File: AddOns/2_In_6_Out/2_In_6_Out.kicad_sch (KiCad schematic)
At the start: 13 parts, among them J1 Heimtime, J2 MasterTrigger, J3 Conn_01x13_Socket, J4 Conn_01x04_Socket, J5 Conn_01x04_Socket

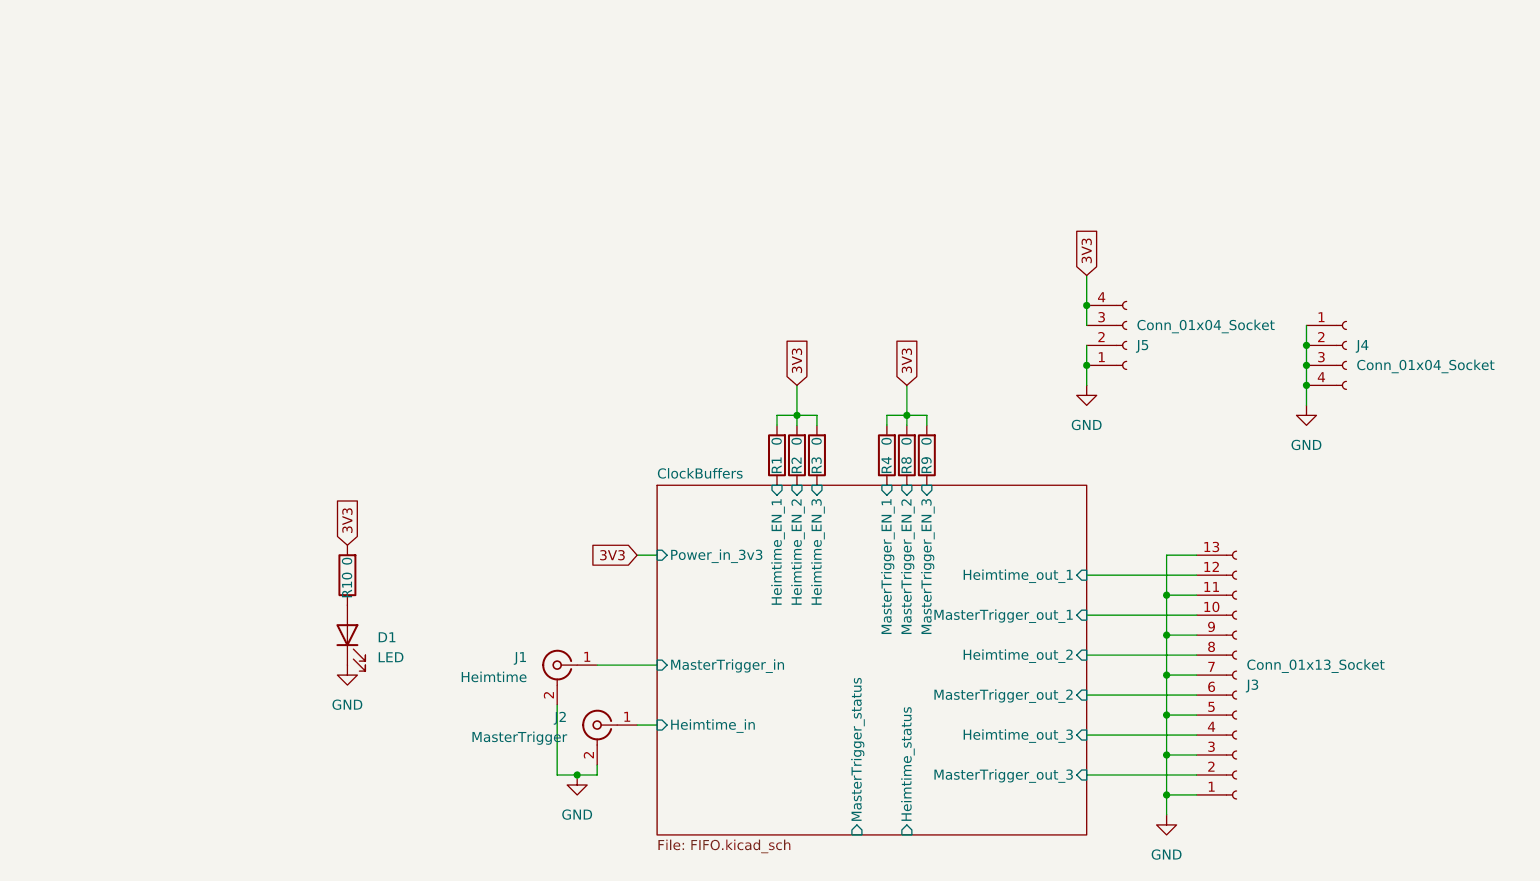
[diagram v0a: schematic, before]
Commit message: .
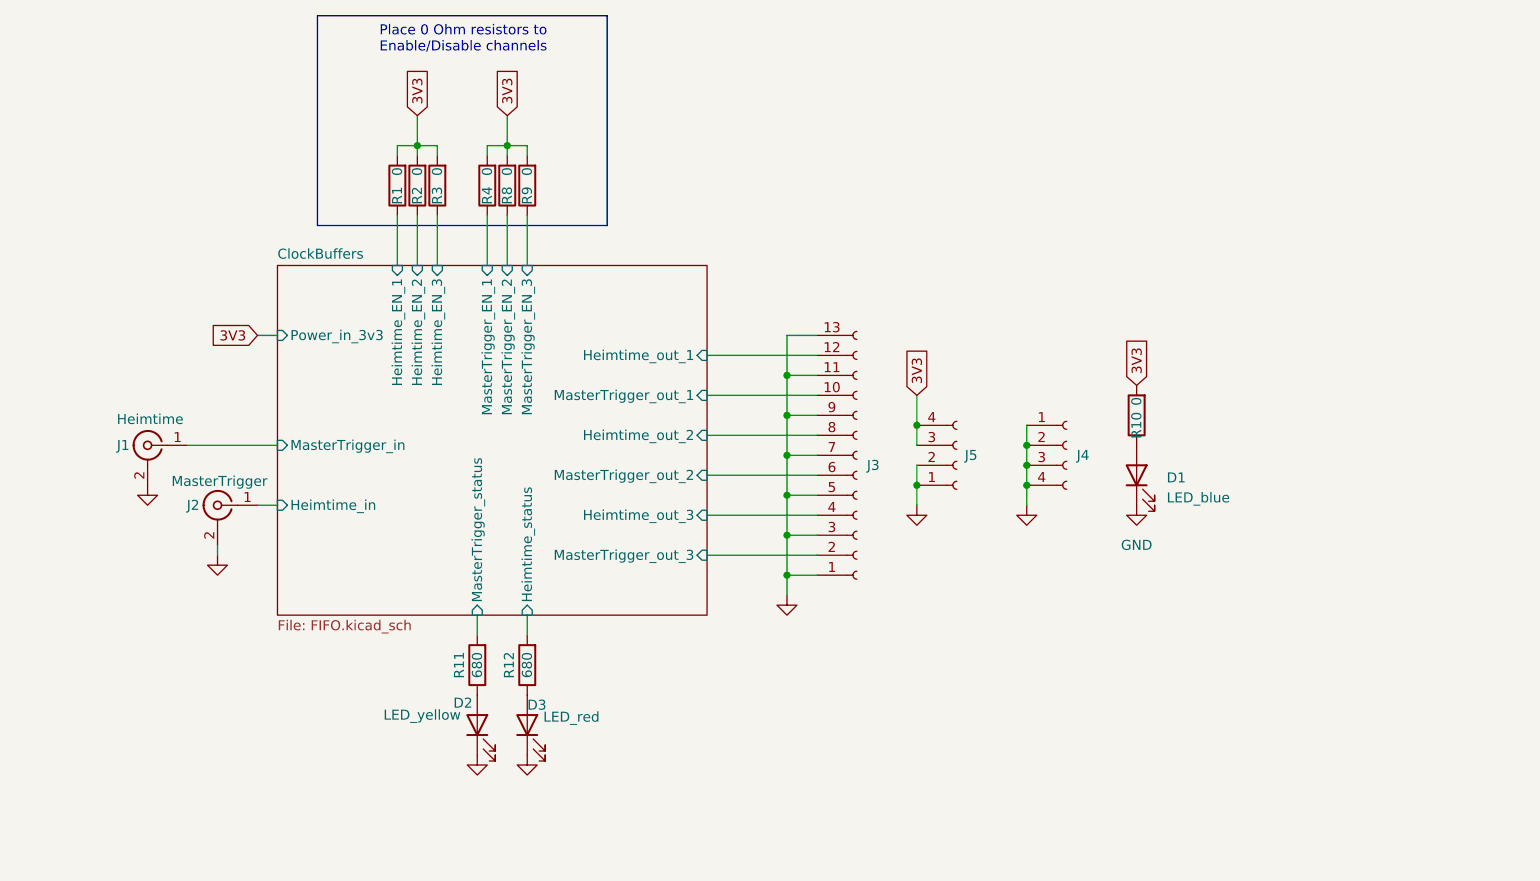
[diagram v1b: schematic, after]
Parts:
- added D2: LED_yellow, LED_SMD:LED_0603_1608Metric, symbol Device:LED
- added D3: LED_red, LED_SMD:LED_0603_1608Metric, symbol Device:LED
- added R11, R12: 680, Resistor_SMD:R_0402_1005Metric, symbol Device:R
- D1: value LED -> LED_blue
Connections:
- net ClockBuffers/Heimtime_status: now also R12.2
- net ClockBuffers/MasterTrigger_status: now also R11.2
- net GND: now also D2.1 (K), D3.1 (K)
- new net: D2.2 (A), R11.1
- new net: D3.2 (A), R12.1
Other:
- note added: "Place 0 Ohm resistors to Enable/Disable channels"
- title: (none) -> Clock Buffers AddOn
- moved on the sheet: D1, J1, J2, J3, J4, J5, R1, R10, R2, R3, R4, R8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

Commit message: .
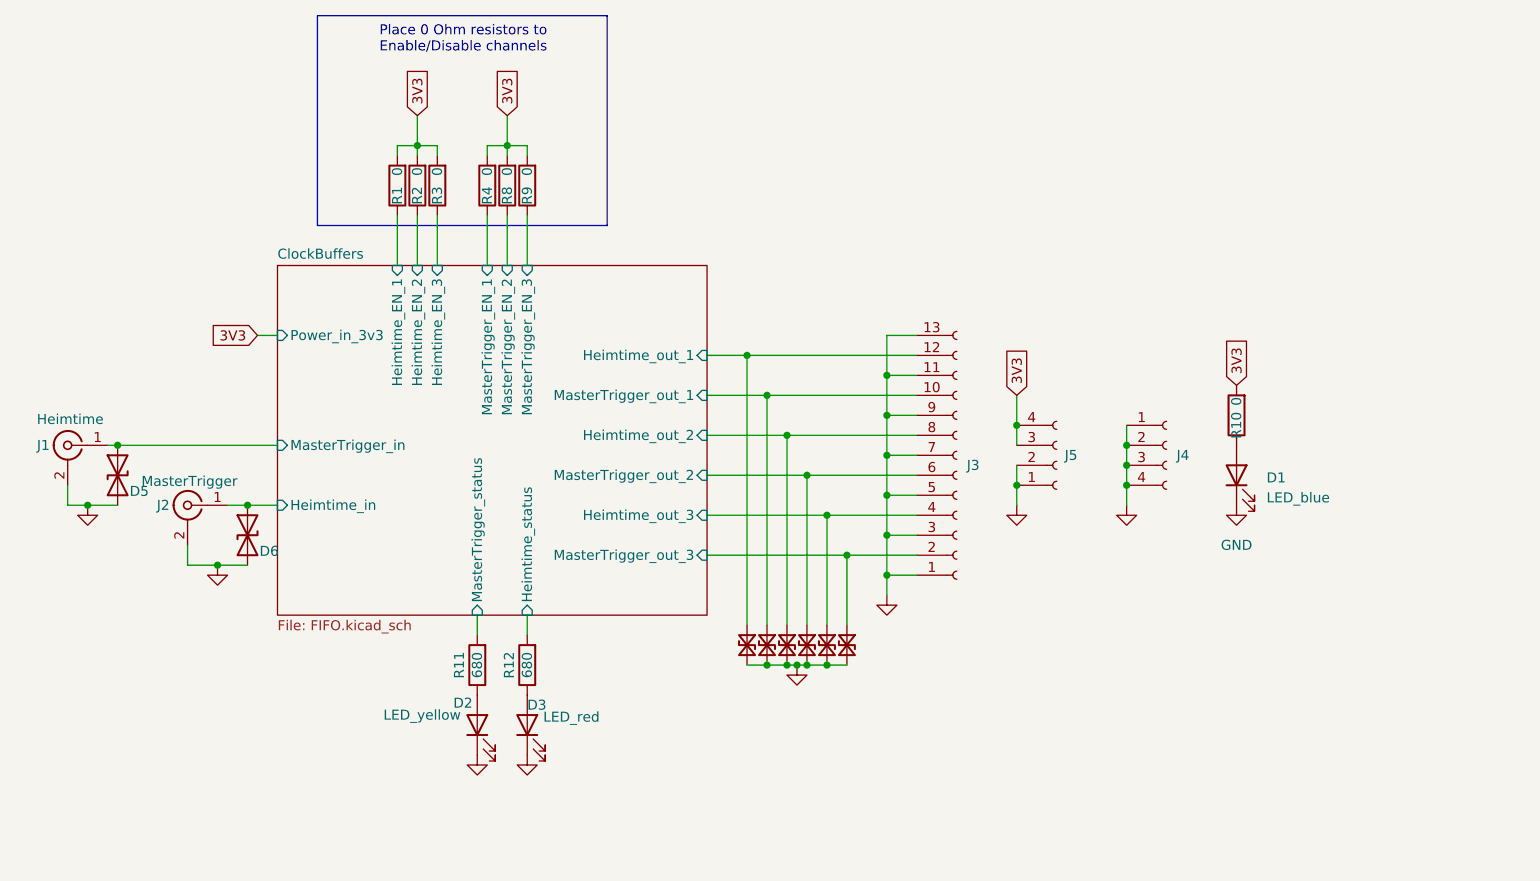
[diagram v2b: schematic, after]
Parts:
- added D10, D11, D13, D7, D8, D9: SP1333-01UTG, Diode_SMD:D_0201_0603Metric, symbol Device:D_TVS_Small
- added D5, D6: SP1333-01UTG, Diode_SMD:D_0201_0603Metric, symbol Device:D_TVS
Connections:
- net ClockBuffers/Heimtime_in: now also D6.1 (A1)
- net ClockBuffers/Heimtime_out_1: now also D13.1 (A1)
- net ClockBuffers/Heimtime_out_2: now also D8.1 (A1)
- net ClockBuffers/Heimtime_out_3: now also D10.1 (A1)
- net ClockBuffers/MasterTrigger_in: now also D5.1 (A1)
- net ClockBuffers/MasterTrigger_out_1: now also D7.1 (A1)
- net ClockBuffers/MasterTrigger_out_2: now also D9.1 (A1)
- net ClockBuffers/MasterTrigger_out_3: now also D11.1 (A1)
- net GND: now also D10.2 (A2), D11.2 (A2), D13.2 (A2), D5.2 (A2), D6.2 (A2), D7.2 (A2), D8.2 (A2), D9.2 (A2)
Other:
- moved on the sheet: D1, J1, J2, J3, J4, J5, R10
